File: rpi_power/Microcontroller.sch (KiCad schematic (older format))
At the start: 12 parts, among them U2 ATxmega16A4U-AU, U3 LM2936-3.3, Y1 Crystal

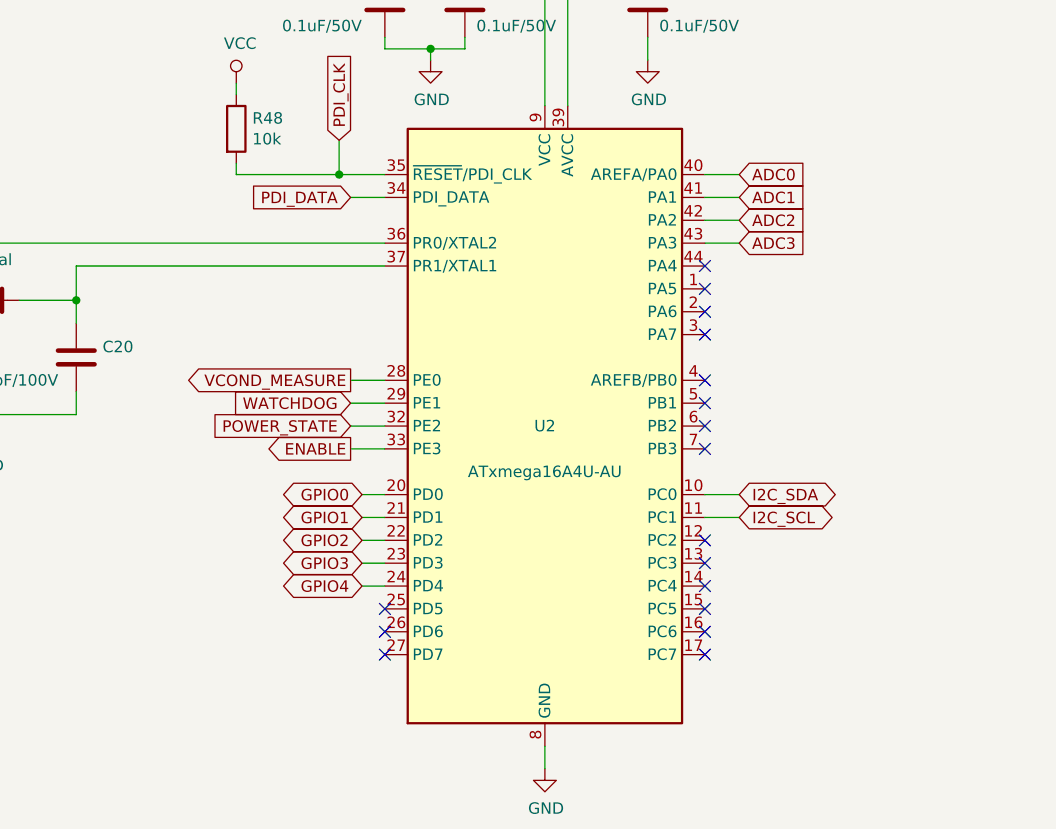
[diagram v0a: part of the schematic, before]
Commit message: Components placed.
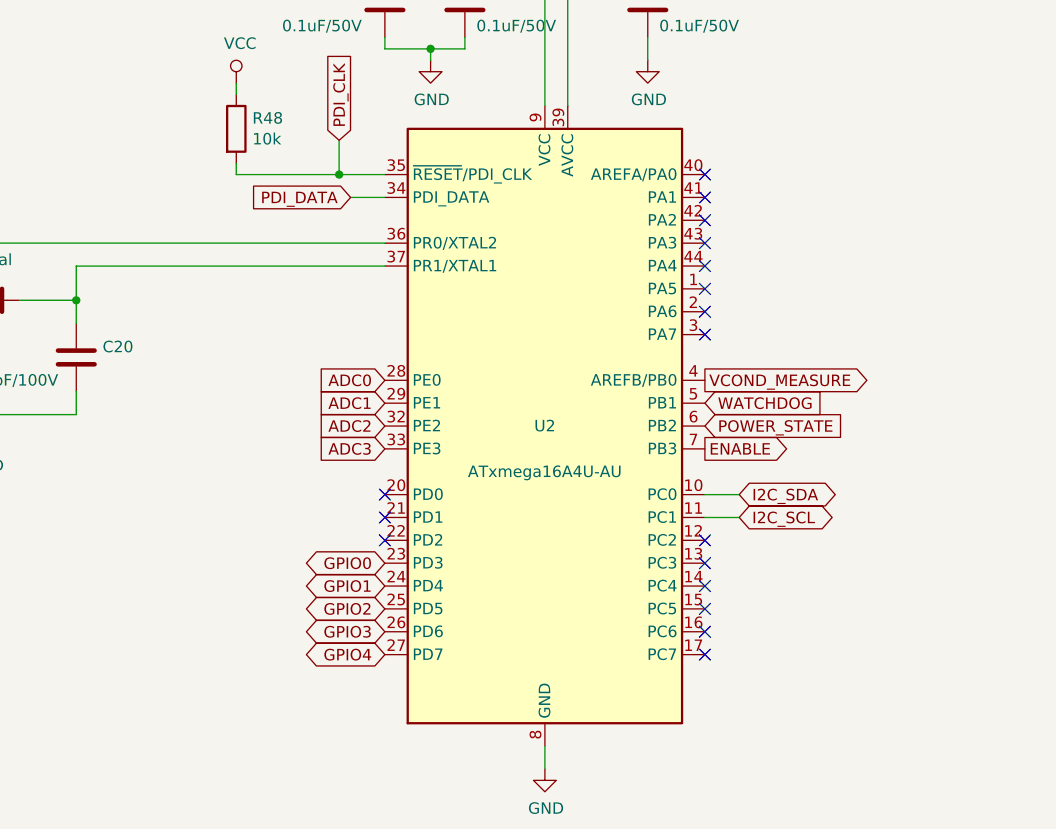
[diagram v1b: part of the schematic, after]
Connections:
- net ADC0: now also U2.28 (PE0); no longer U2.40 (AREFA/PA0)
- net ADC1: now also U2.29 (PE1); no longer U2.41 (PA1)
- net ADC2: now also U2.32 (PE2); no longer U2.42 (PA2)
- net ADC3: now also U2.33 (PE3); no longer U2.43 (PA3)
- net ENABLE: now also U2.7 (PB3); no longer U2.33 (PE3)
- net GPIO0: now also U2.23 (PD3); no longer U2.20 (PD0)
- net GPIO1: now also U2.24 (PD4); no longer U2.21 (PD1)
- net GPIO2: now also U2.25 (PD5); no longer U2.22 (PD2)
- net GPIO3: now also U2.26 (PD6); no longer U2.23 (PD3)
- net GPIO4: now also U2.27 (PD7); no longer U2.24 (PD4)
- net POWER_STATE: now also U2.6 (PB2); no longer U2.32 (PE2)
- net VCOND_MEASURE: now also U2.4 (AREFB/PB0); no longer U2.28 (PE0)
- net WATCHDOG: now also U2.5 (PB1); no longer U2.29 (PE1)
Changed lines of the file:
@@
 Wire Wire Line
 	4650 3850 4800 3850
-Wire Wire Line
-	4650 2350 4800 2350
-Wire Wire Line
-	4650 2450 4800 2450
-Wire Wire Line
-	4650 2550 4800 2550
-Wire Wire Line
-	4650 2650 4800 2650
-Wire Wire Line
-	3250 3250 3100 3250
-Wire Wire Line
-	3250 3350 3100 3350
-Wire Wire Line
-	3250 3450 3100 3450
-Wire Wire Line
-	3250 3550 3100 3550
-Text GLabel 3100 3550 0    50   Output ~ 0
+Text GLabel 4650 3550 2    50   Output ~ 0
 ENABLE
-Text GLabel 3100 3250 0    50   Output ~ 0
+Text GLabel 4650 3250 2    50   Output ~ 0
 VCOND_MEASURE
-Text GLabel 3100 3450 0    50   Input ~ 0
+Text GLabel 4650 3450 2    50   Input ~ 0
 POWER_STATE
-Text GLabel 3100 3350 0    50   Input ~ 0
+Text GLabel 4650 3350 2    50   Input ~ 0
 WATCHDOG
-Text GLabel 4800 2350 2    50   Input ~ 0
+Text GLabel 3250 3250 0    50   Input ~ 0
 ADC0
-Text GLabel 4800 2450 2    50   Input ~ 0
+Text GLabel 3250 3350 0    50   Input ~ 0
 ADC1
-Text GLabel 4800 2550 2    50   Input ~ 0
+Text GLabel 3250 3450 0    50   Input ~ 0
 ADC2
-Text GLabel 4800 2650 2    50   Input ~ 0
+Text GLabel 3250 3550 0    50   Input ~ 0
 ADC3
 Text GLabel 4800 3750 2    50   BiDi ~ 0
@@
 Wire Wire Line
 	4200 1400 4400 1400
-Wire Wire Line
-	3150 3750 3250 3750
-Wire Wire Line
-	3150 3850 3250 3850
-Wire Wire Line
-	3150 3950 3250 3950
-Wire Wire Line
-	3150 4050 3250 4050
-Wire Wire Line
-	3150 4150 3250 4150
 NoConn ~ 4650 2750
 NoConn ~ 4650 2850
 NoConn ~ 4650 2950
 NoConn ~ 4650 3050
-NoConn ~ 4650 3250
-NoConn ~ 4650 3350
-NoConn ~ 4650 3450
-NoConn ~ 4650 3550
 NoConn ~ 4650 3950
 NoConn ~ 4650 4050
@@
 Text GLabel 3050 2200 1    50   Input ~ 0
 PDI_CLK
-Text GLabel 3150 3750 0    50   BiDi ~ 0
+Text GLabel 3250 4050 0    50   BiDi ~ 0
 GPIO0
-Text GLabel 3150 3850 0    50   BiDi ~ 0
+Text GLabel 3250 4150 0    50   BiDi ~ 0
 GPIO1
-Text GLabel 3150 3950 0    50   BiDi ~ 0
+Text GLabel 3250 4250 0    50   BiDi ~ 0
 GPIO2
-Text GLabel 3150 4050 0    50   BiDi ~ 0
+Text GLabel 3250 4350 0    50   BiDi ~ 0
 GPIO3
-Text GLabel 3150 4150 0    50   BiDi ~ 0
+Text GLabel 3250 4450 0    50   BiDi ~ 0
 GPIO4
-NoConn ~ 3250 4250
-NoConn ~ 3250 4350
-NoConn ~ 3250 4450
+NoConn ~ 3250 3750
+NoConn ~ 3250 3850
+NoConn ~ 3250 3950
+NoConn ~ 4650 2350
+NoConn ~ 4650 2450
+NoConn ~ 4650 2550
+NoConn ~ 4650 2650
 $EndSCHEMATC
